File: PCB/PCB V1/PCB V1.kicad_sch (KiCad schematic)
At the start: 50 parts, among them J1 Screw_Terminal_01x03, J2 Screw_Terminal_01x03, J3 USB_B, J4 Conn_01x02_Pin, K1 Relay_SPDT, K2 Relay_SPDT, Q1 S8050, Q2 S8050, Q3 S8050, SW1 On/Off, SW2 SW_Push, SW3 SW_Push, U1 LM317_TO-220

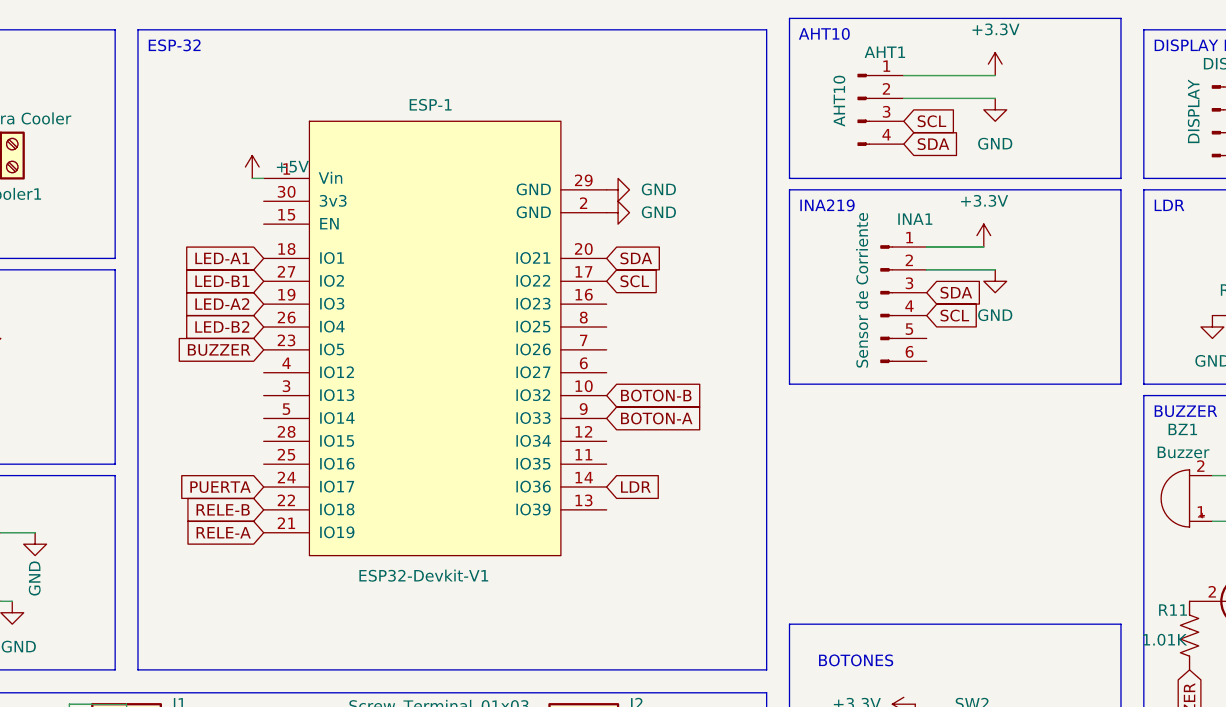
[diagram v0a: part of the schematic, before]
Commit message: .
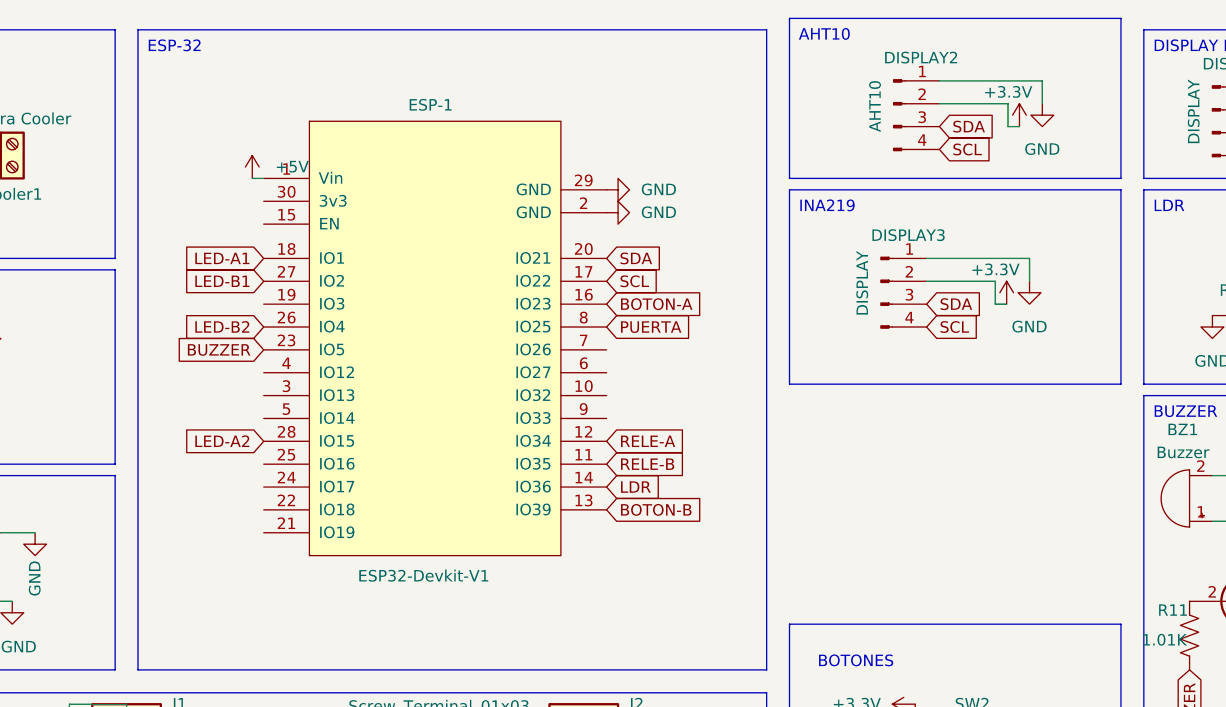
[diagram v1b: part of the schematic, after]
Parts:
- removed AHT1: AHT10, Connector_Molex:Molex_KK-254_AE-6410-04A_1x04_P2.54mm_Vertical, symbol Connector:Conn_01x04_Pin
- removed INA1: Sensor de Corriente, Connector_PinHeader_2.54mm:PinHeader_1x06_P2.54mm_Vertical, symbol Connector:Conn_01x06_Pin
- added DISPLAY2: AHT10, Connector_Molex:Molex_KK-254_AE-6410-04A_1x04_P2.54mm_Vertical, symbol Connector:Conn_01x04_Pin
- added DISPLAY3: DISPLAY, Connector_Molex:Molex_KK-254_AE-6410-04A_1x04_P2.54mm_Vertical, symbol Connector:Conn_01x04_Pin
- D5, D7: footprint Connector_Molex:Molex_KK-254_AE-6410-02A_1x02_P2.54mm_Vertical -> LED_THT:LED_D5.0mm_Clear
- J4: footprint Connector_PinHeader_2.54mm:PinHeader_1x02_P2.54mm_Vertical -> Connector_Molex:Molex_KK-254_AE-6410-02A_1x02_P2.54mm_Vertical
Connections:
- net +3.3V: now also DISPLAY2.2 (Pin_2), DISPLAY3.2 (Pin_2)
- net BOTON-A: now also ESP-1.16 (IO23); no longer ESP-1.9 (IO33)
- net BOTON-B: now also ESP-1.13 (IO39); no longer ESP-1.10 (IO32)
- net GND: now also DISPLAY2.1 (Pin_1), DISPLAY3.1 (Pin_1)
- net LED-A2: now also ESP-1.28 (IO15); no longer ESP-1.19 (IO3)
- net PUERTA: now also ESP-1.8 (IO25); no longer ESP-1.24 (IO17)
- net RELE-A: now also ESP-1.12 (IO34); no longer ESP-1.21 (IO19)
- net RELE-B: now also ESP-1.11 (IO35); no longer ESP-1.22 (IO18)
- net SCL: now also DISPLAY2.4 (Pin_4), DISPLAY3.4 (Pin_4)
- net SDA: now also DISPLAY2.3 (Pin_3), DISPLAY3.3 (Pin_3)

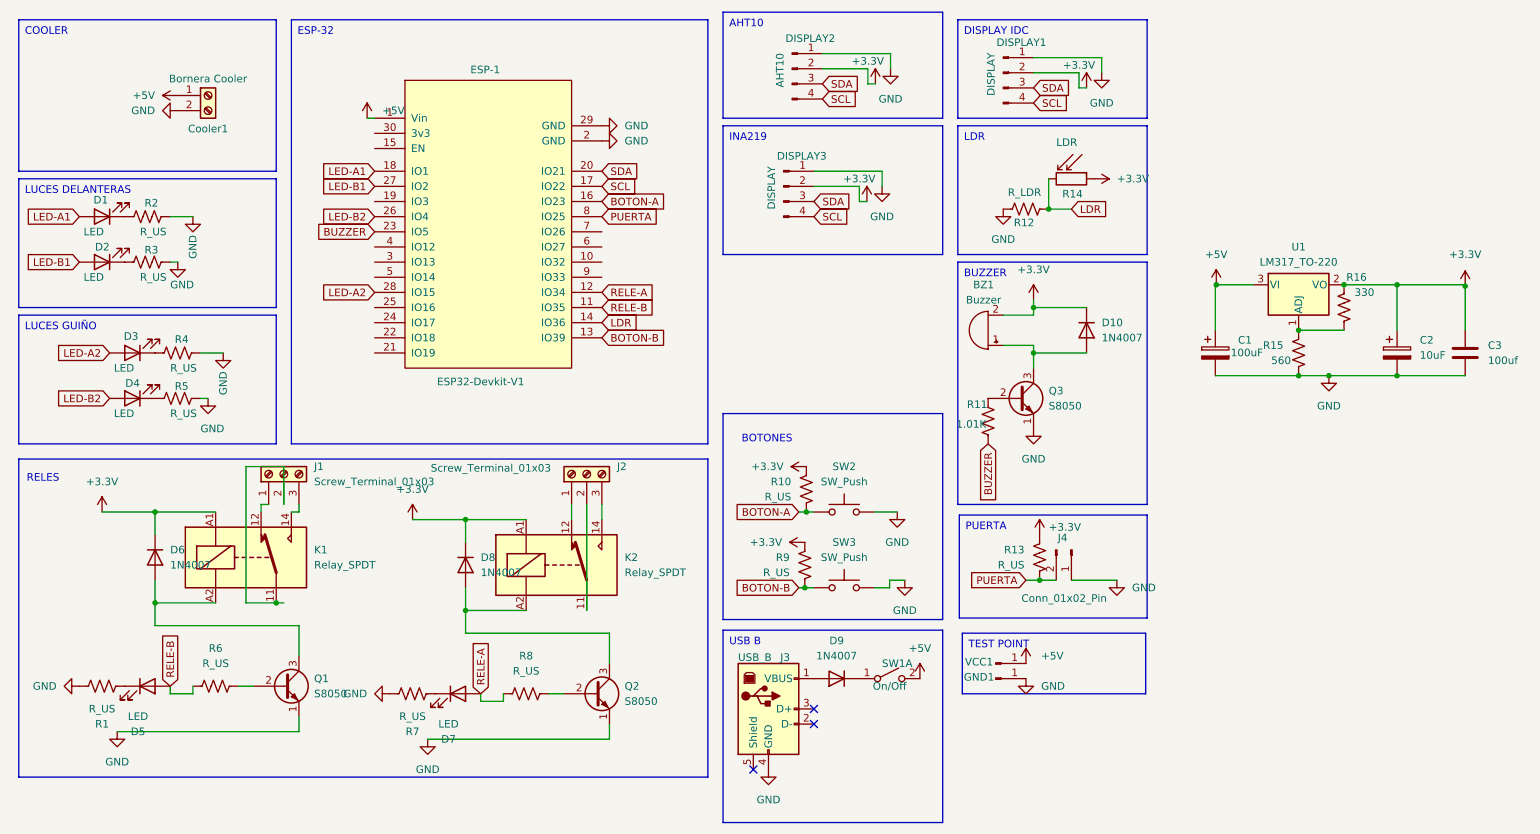
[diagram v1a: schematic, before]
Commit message: .
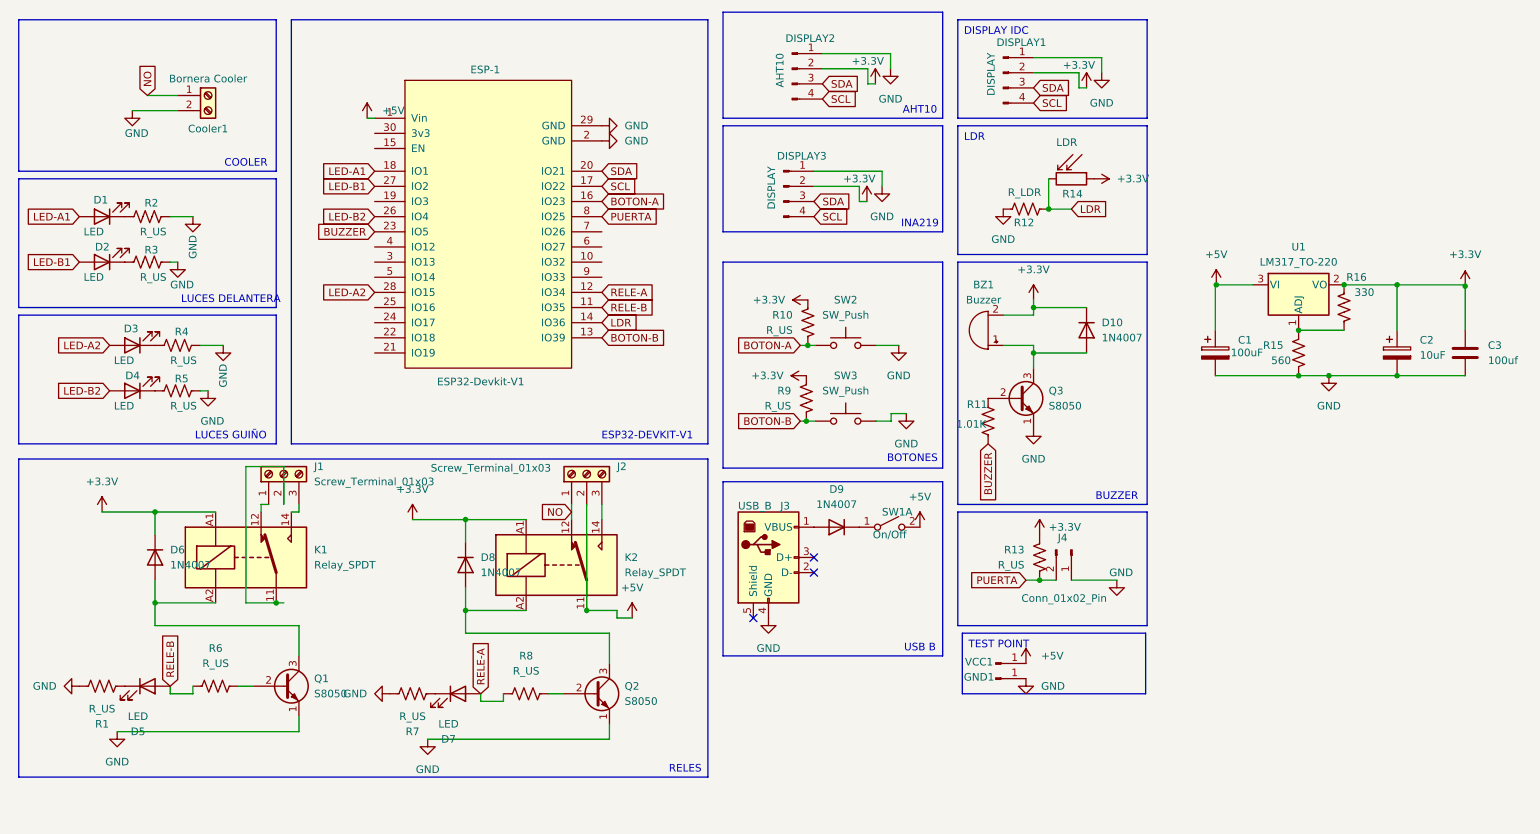
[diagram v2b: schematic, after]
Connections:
- net +5V: now also J2.2 (Pin_2), K2.11; no longer Cooler1.1 (Pin_1)
- net NO: now reaches J2.1 (Pin_1), K2.12
- net NO: now also Cooler1.1 (Pin_1)
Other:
- note added: "AHT10"
- note added: "BUZZER"
- note added: "COOLER"
- note added: "ESP32-DEVKIT-V1"
- note added: "INA219"
- note added: "LUCES DELANTERA"
- note added: "LUCES GUIÑO"
- note added: "USB B"
- moved on the sheet: D3, D4, D9, J3, R10, R4, R5, R9, SW1A, SW2, SW3
